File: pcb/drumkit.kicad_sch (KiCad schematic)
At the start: 22 parts, among them IC1 ULN2065B, J1 BATTERY, J2 Conn_01x04_Female, J3 CH1, J4 CH2, J5 CH3, SW1 BUTTON1, SW2 BUTTON2, SW3 BUTTON3, SW4 BUTTON4, SW5 POWER_SW, U1 Pico, U2 Mini360

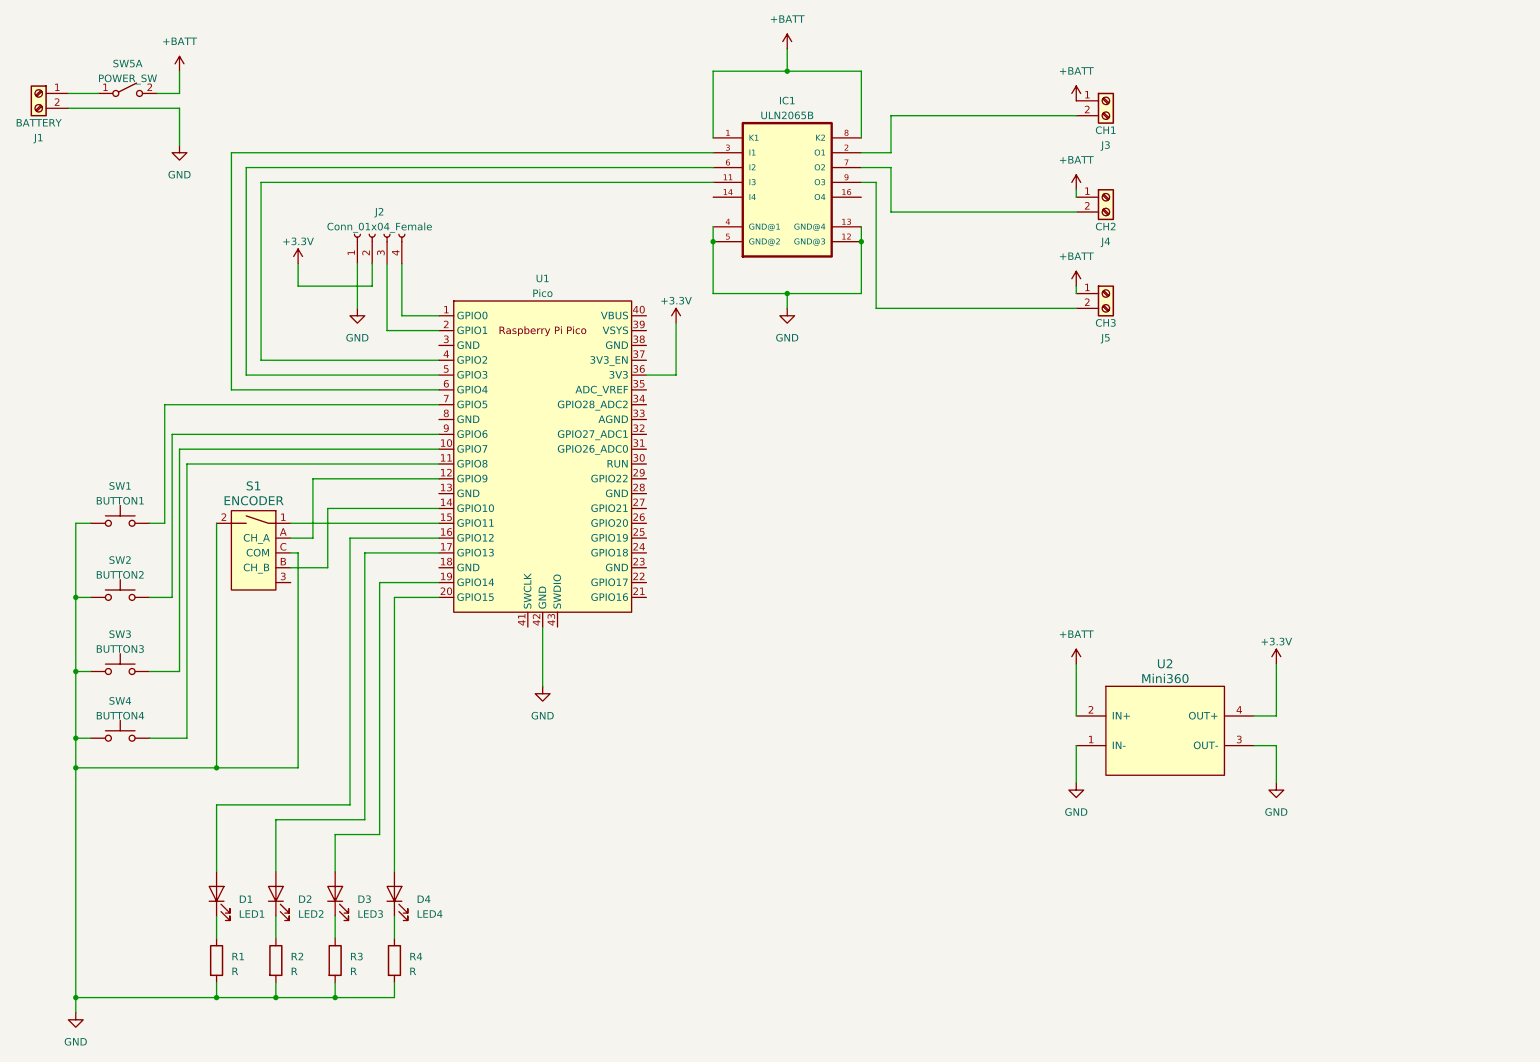
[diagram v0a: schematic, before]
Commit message: fix board
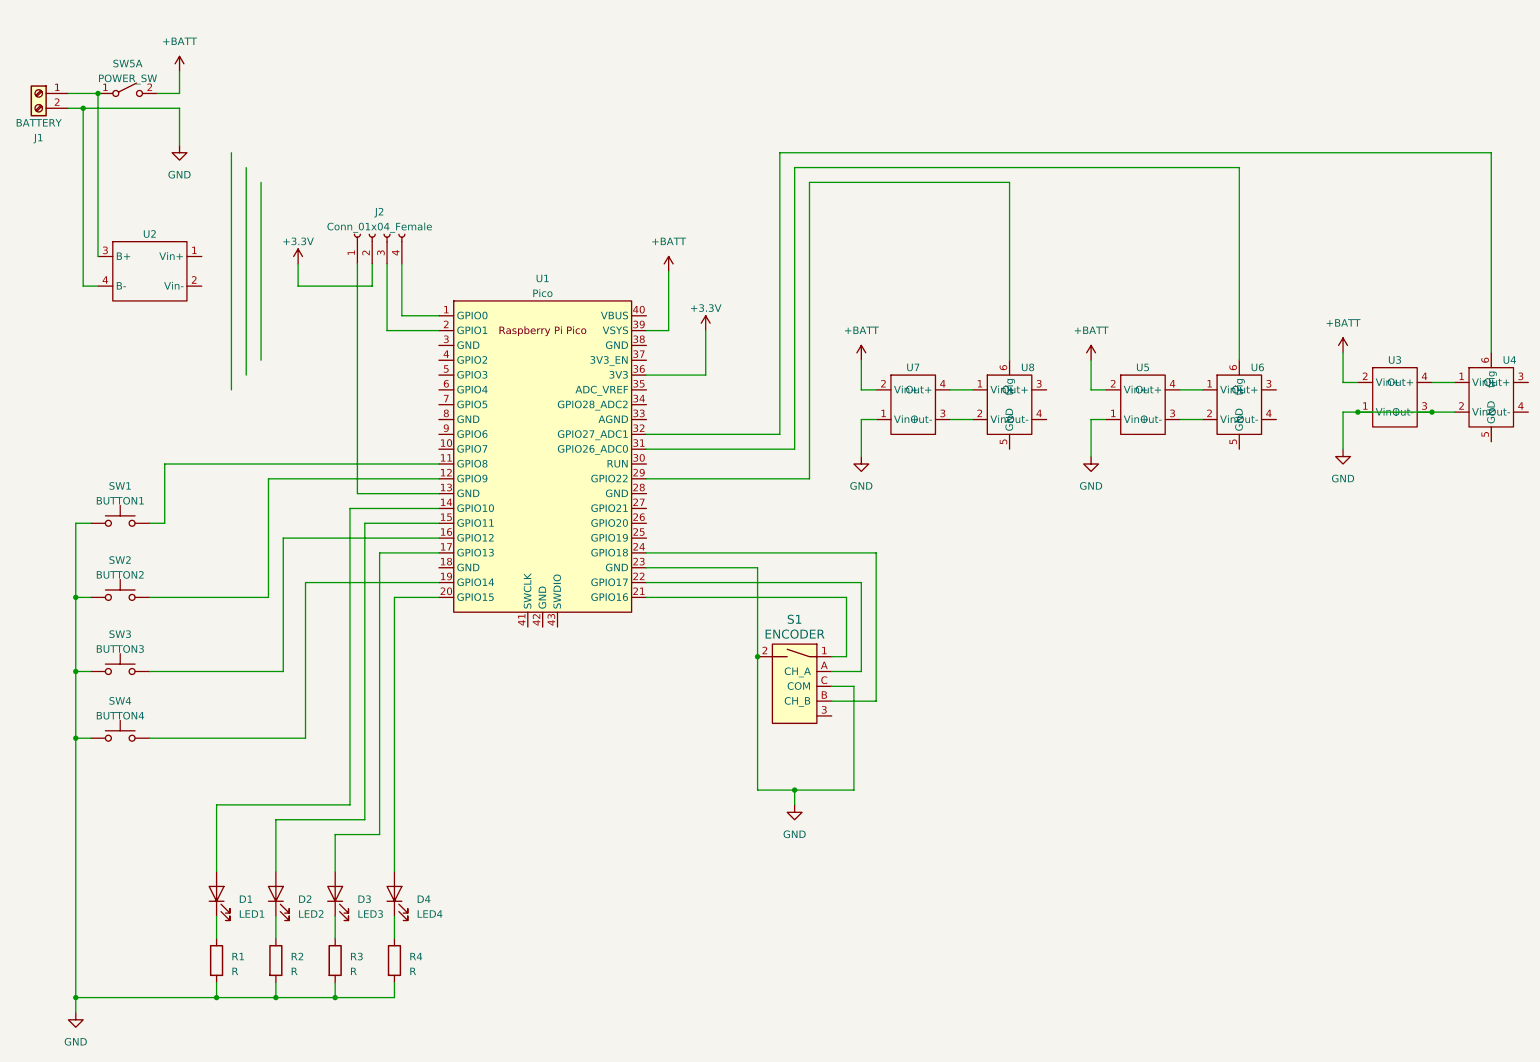
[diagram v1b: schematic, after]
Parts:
- removed IC1: ULN2065B, Package_DIP:DIP-16_W7.62mm_LongPads, symbol ULN2065B:ULN2065B
- removed J3: CH1, TerminalBlock:TerminalBlock_bornier-2_P5.08mm, symbol Connector:Screw_Terminal_01x02
- removed J4: CH2, TerminalBlock:TerminalBlock_bornier-2_P5.08mm, symbol Connector:Screw_Terminal_01x02
- removed J5: CH3, TerminalBlock:TerminalBlock_bornier-2_P5.08mm, symbol Connector:Screw_Terminal_01x02
- removed U2: Mini360, Mini360_step-down:Mini360_step-down, symbol mini360:Mini360
- added U2: ~, chinese_modules:charger, symbol chinese_modules:charger
- added U3, U5, U7: ~, chinese_modules:dc-dc module, symbol chinese_modules:dc-dc
- added U4, U6, U8: ~, chinese_modules:xy-mos, symbol chinese_modules:xy-mos
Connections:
- net +BATT: now also U1.39 (VSYS), U3.2 (Vin+), U5.2 (Vin+), U7.2 (Vin+)
- net GND: now also U1.23 (GND), U2.4 (B-), U3.1 (Vin+), U3.3 (Out-), U4.2 (Vin-), U5.1 (Vin+), U7.1 (Vin+); no longer J2.1 (Pin_1), U1.42 (GND)
- net at U1.15 (GPIO11): now also D2.2 (A); no longer S1.1
- net at U1.12 (GPIO9): now also SW2.2; no longer S1.A (CH_A)
- net at S1.B (CH_B): now also U1.24 (GPIO18); no longer U1.14 (GPIO10)
- net at D3.2 (A): now also U1.17 (GPIO13); no longer U1.19 (GPIO14)
- net at J1.1 (Pin_1), SW5.1 (A): now also U2.3 (B+)
- net at SW1.2: now also U1.11 (GPIO8); no longer U1.7 (GPIO5)
- net at U1.9 (GPIO6): no longer SW2.2
- net at SW3.2: now also U1.16 (GPIO12); no longer U1.10 (GPIO7)
- net at SW4.2: now also U1.19 (GPIO14); no longer U1.11 (GPIO8)
- net at U1.13 (GND): now also J2.1 (Pin_1)
- net at D1.2 (A): now also U1.14 (GPIO10); no longer U1.16 (GPIO12)
- net at U1.21 (GPIO16): now also S1.1
- net at U1.22 (GPIO17): now also S1.A (CH_A)
- net at U1.29 (GPIO22): now also U8.6 (trig)
- net at U1.31 (GPIO26_ADC0): now also U6.6 (trig)
- net at U1.32 (GPIO27_ADC1): now also U4.6 (trig)
- new net: U7.4 (Out+), U8.1 (Vin+)
- new net: U7.3 (Out-), U8.2 (Vin-)
- new net: U5.3 (Out-), U6.2 (Vin-)
- new net: U5.4 (Out+), U6.1 (Vin+)
- new net: U3.4 (Out+), U4.1 (Vin+)
